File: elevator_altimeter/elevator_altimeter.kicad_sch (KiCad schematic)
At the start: 44 parts, among them J1 UART, J2 AVR-ICSP-TagConnect, J3 I2C, SW1 UserSW, U1 MPL3115A2, U2 NRF24L01_Breakout, U3 ATtiny1634-S, U4 MCP1711, U5 TP4056

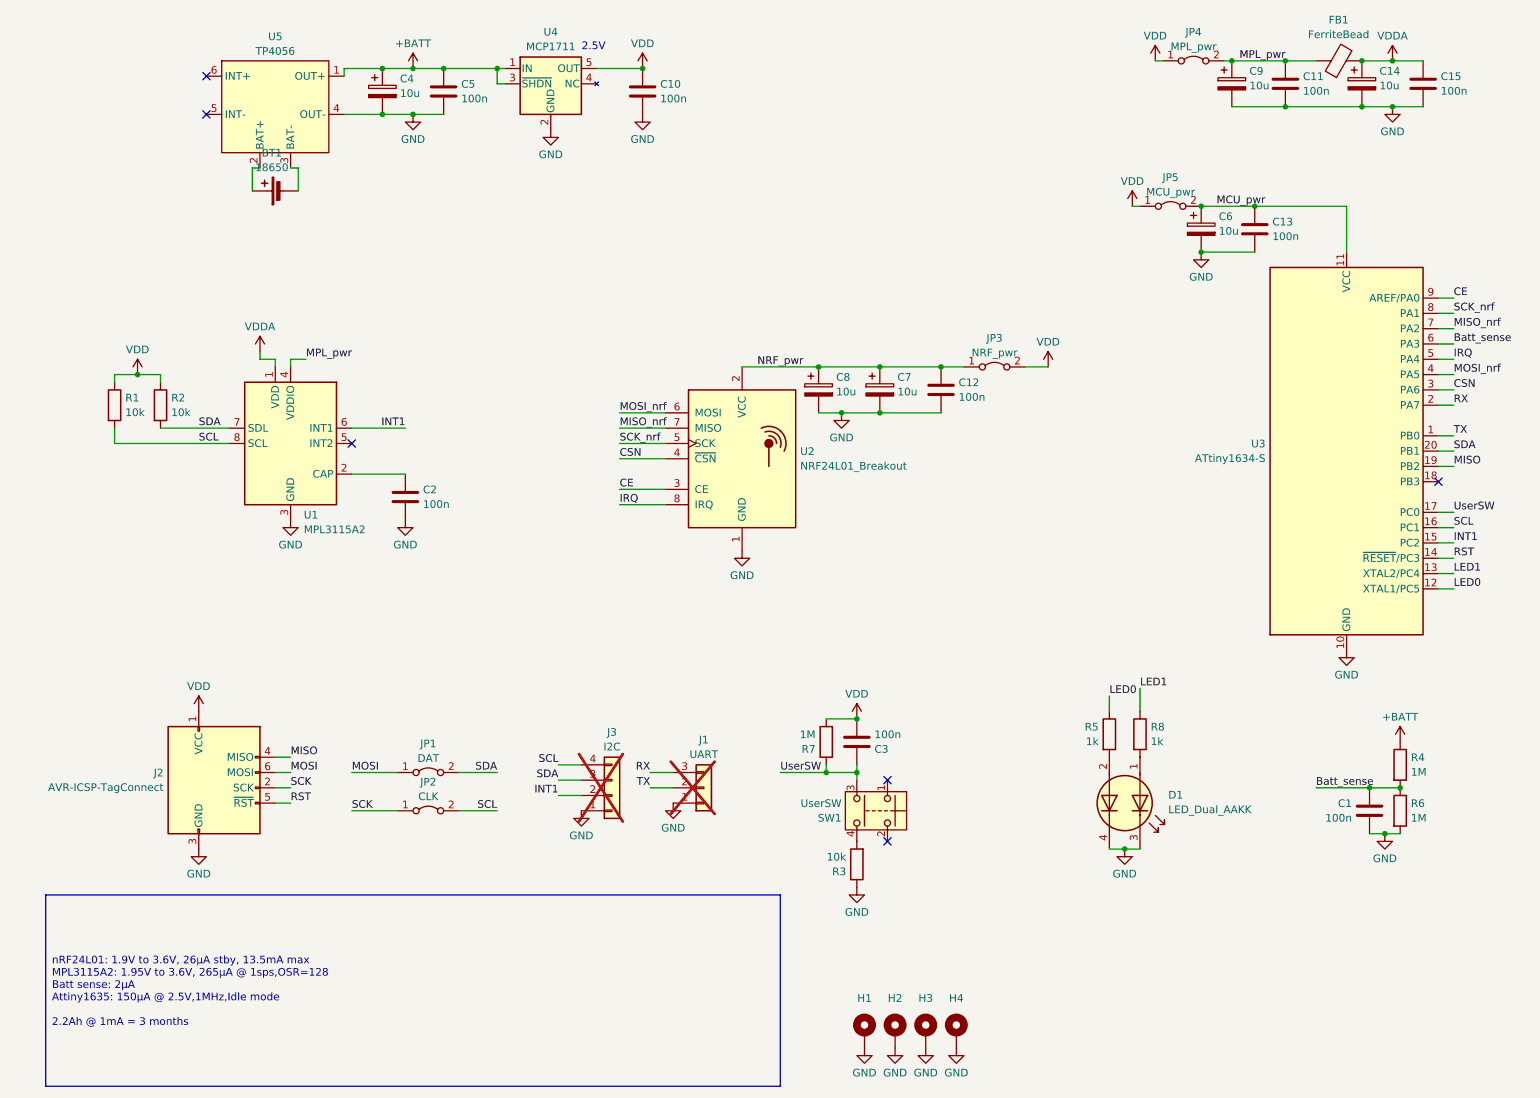
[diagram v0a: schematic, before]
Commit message: a
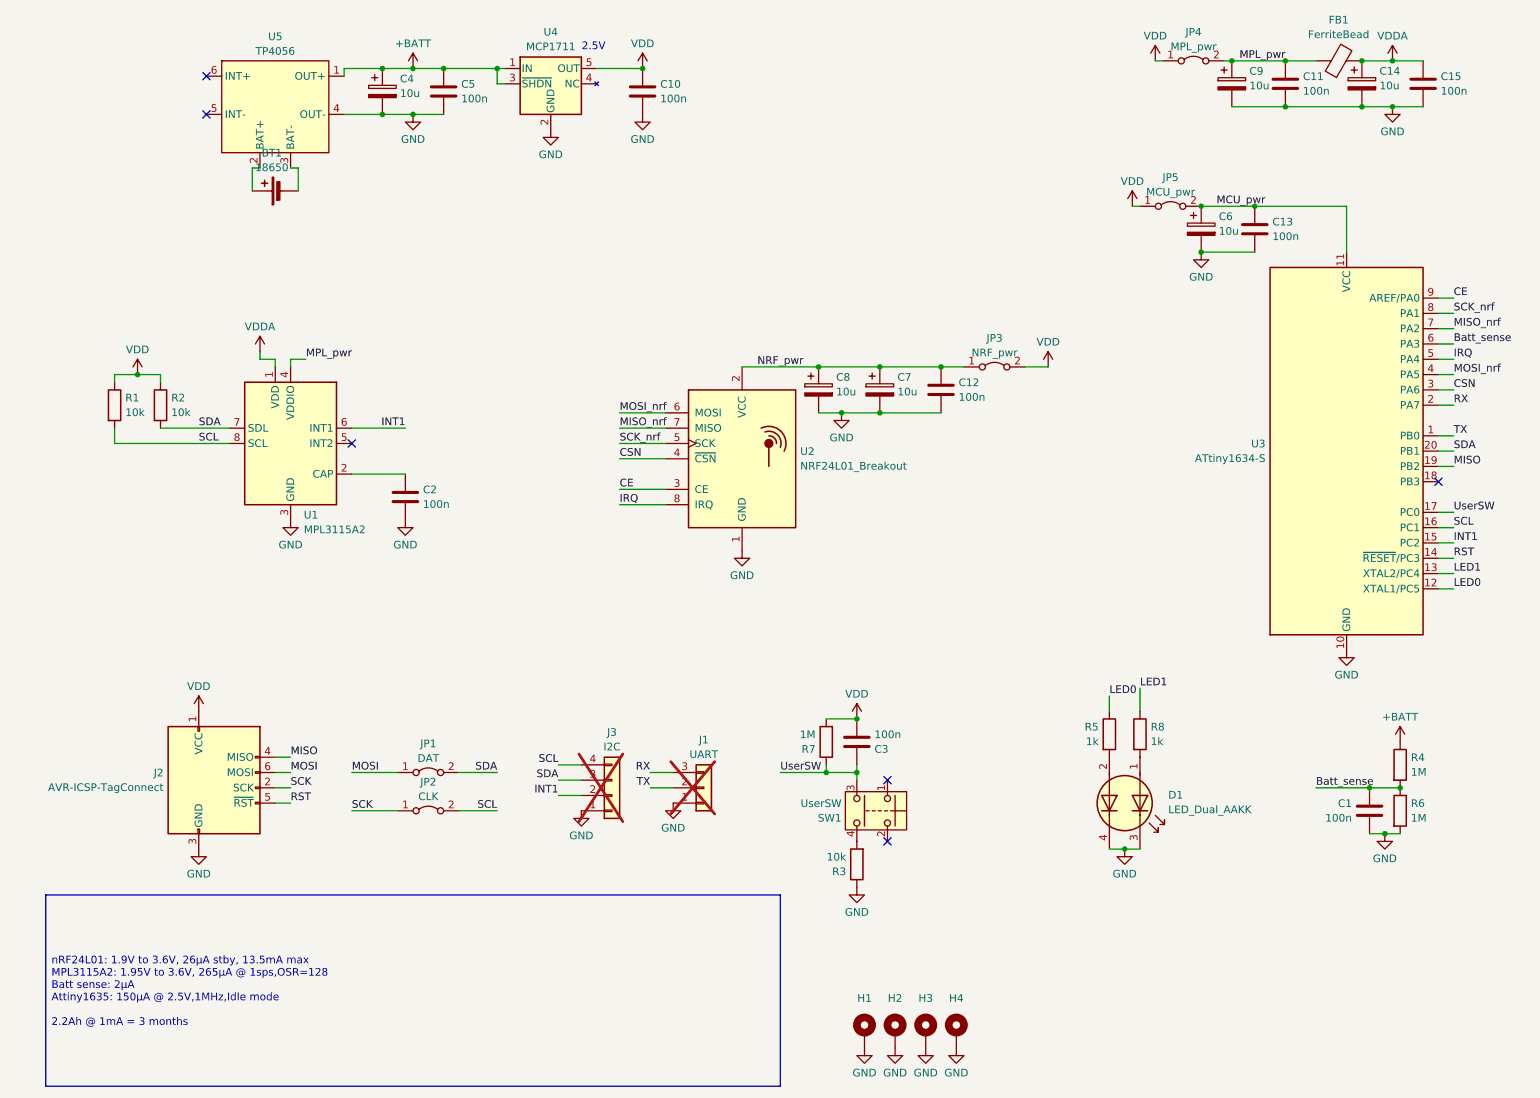
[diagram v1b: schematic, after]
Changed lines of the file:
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@@
 (kicad_sch
-	(version 20231120)
+	(version 20250114)
 	(generator "eeschema")
-	(generator_version "8.0")
+	(generator_version "9.0")
 	(paper "A4")
 	(title_block
@@
 		(company "Xavier Bourlot")
 	)
+	(text "2.5V"
+		(exclude_from_sim no)
+		(at 108.712 20.574 0)
+		(effects
+			(font
+				(size 1.27 1.27)
+			)
+		)
+	)
+	(text_box "nRF24L01: 1.9V to 3.6V, 26µA stby, 13.5mA max\nMPL3115A2: 1.95V to 3.6V, 265µA @ 1sps,OSR=128\nBatt sense: 2µA\nAttiny1635: 150µA @ 2.5V,1MHz,Idle mode\n\n2.2Ah @ 1mA = 3 months"
+		(exclude_from_sim no)
+		(at 17.78 161.29 0)
+		(size 121.92 31.75)
+		(margins 0.9525 0.9525 0.9525 0.9525)
+		(stroke
+			(width 0)
+			(type default)
+		)
+		(fill
+			(type color)
+			(color 255 255 194 1)
+		)
+		(effects
+			(font
+				(size 1.27 1.27)
+			)
+			(justify left)
+		)
+	)
 	(junction
 		(at 152.4 132.08)
@@
 		)
 	)
-	(text_box "nRF24L01: 1.9V to 3.6V, 26µA stby, 13.5mA max\nMPL3115A2: 1.95V to 3.6V, 265µA @ 1sps,OSR=128\nBatt sense: 2µA\nAttiny1635: 150µA @ 2.5V,1MHz,Idle mode\n\n2.2Ah @ 1mA = 3 months"
-		(exclude_from_sim no)
-		(at 17.78 161.29 0)
-		(size 121.92 31.75)
-		(stroke
-			(width 0)
-			(type default)
-		)
-		(fill
-			(type color)
-			(color 255 255 194 1)
-		)
-		(effects
-			(font
-				(size 1.27 1.27)
-			)
-			(justify left)
-		)
-	)
-	(text "2.5V"
-		(exclude_from_sim no)
-		(at 108.712 20.574 0)
-		(effects
-			(font
-				(size 1.27 1.27)
-			)
-		)
-	)
 	(label "SCL"
 		(at 251.46 100.33 0)
-		(fields_autoplaced yes)
 		(effects
 			(font
@@
 	(label "RX"
 		(at 251.46 80.01 0)
-		(fields_autoplaced yes)
 		(effects
 			(font
@@
 	(label "CE"
 		(at 251.46 62.23 0)
-		(fields_autoplaced yes)
 		(effects
 			(font
@@
 	(label "SDA"
 		(at 102.87 142.24 180)
-		(fields_autoplaced yes)
 		(effects
 			(font
@@
 	(label "MISO_nrf"
 		(at 113.03 83.82 0)
-		(fields_autoplaced yes)
 		(effects
 			(font
@@
 	(label "INT1"
 		(at 77.47 83.82 180)
-		(fields_autoplaced yes)
 		(effects
 			(font
@@
 	(label "SDA"
 		(at 92.71 140.97 180)
-		(fields_autoplaced yes)
 		(effects
 			(font
@@
 	(label "SCL"
 		(at 102.87 139.7 180)
-		(fields_autoplaced yes)
 		(effects
 			(font
@@
 	(label "MOSI_nrf"
 		(at 251.46 74.93 0)
-		(fields_autoplaced yes)
 		(effects
 			(font
@@
 	(label "MCU_pwr"
 		(at 212.09 46.99 0)
-		(fields_autoplaced yes)
 		(effects
 			(font
@@
 	(label "MPL_pwr"
 		(at 60.96 72.39 0)
-		(fields_autoplaced yes)
 		(effects
 			(font
@@
 	(label "LED1"
 		(at 251.46 107.95 0)
-		(fields_autoplaced yes)
 		(effects
 			(font
@@
 	(label "SCL"
 		(at 43.18 86.36 0)
-		(fields_autoplaced yes)
 		(effects
 			(font
@@
 	(label "TX"
 		(at 118.11 143.51 180)
-		(fields_autoplaced yes)
 		(effects
 			(font
@@
 	(label "MOSI"
 		(at 58.42 140.97 0)
-		(fields_autoplaced yes)
 		(effects
 			(font
@@
 	(label "Batt_sense"
 		(at 251.46 69.85 0)
-		(fields_autoplaced yes)
 		(effects
 			(font
@@
 	(label "LED0"
 		(at 251.46 110.49 0)
-		(fields_autoplaced yes)
 		(effects
 			(font
@@
 	(label "MISO"
 		(at 251.46 90.17 0)
-		(fields_autoplaced yes)
 		(effects
 			(font
@@
 	(label "RST"
 		(at 251.46 105.41 0)
-		(fields_autoplaced yes)
 		(effects
 			(font
@@
 	(label "SCK"
 		(at 68.58 147.32 0)
-		(fields_autoplaced yes)
 		(effects
 			(font
@@
 	(label "SCK"
 		(at 58.42 143.51 0)
-		(fields_autoplaced yes)
 		(effects
 			(font
@@
 	(label "MISO"
 		(at 58.42 138.43 0)
-		(fields_autoplaced yes)
 		(effects
 			(font
@@
 	(label "CE"
 		(at 113.03 93.98 0)
-		(fields_autoplaced yes)
 		(effects
 			(font
@@
 	(label "SCK_nrf"
 		(at 113.03 86.36 0)
-		(fields_autoplaced yes)
 		(effects
 			(font
@@
 	(label "RX"
 		(at 118.11 140.97 180)
-		(fields_autoplaced yes)
 		(effects
 			(font
@@
 	(label "MOSI_nrf"
 		(at 113.03 81.28 0)
-		(fields_autoplaced yes)
 		(effects
 			(font
@@
 	(label "Batt_sense"
 		(at 228.6 143.51 0)
-		(fields_autoplaced yes)
 		(effects
 			(font
@@
 	(label "RST"
 		(at 58.42 146.05 0)
-		(fields_autoplaced yes)
 		(effects
 			(font
@@
 	(label "SDA"
 		(at 43.18 83.82 0)
-		(fields_autoplaced yes)
 		(effects
 			(font
@@
 	(label "UserSW"
 		(at 251.46 97.79 0)
-		(fields_autoplaced yes)
 		(effects
 			(font
@@
 	(label "MOSI"
 		(at 68.58 140.97 0)
-		(fields_autoplaced yes)
 		(effects
 			(font
@@
 	(label "UserSW"
 		(at 139.7 140.97 0)
-		(fields_autoplaced yes)
 		(effects
 			(font
@@
 	(label "CSN"
 		(at 251.46 77.47 0)
-		(fields_autoplaced yes)
 		(effects
 			(font
@@
 	(label "NRF_pwr"
 		(at 135.89 73.66 0)
-		(fields_autoplaced yes)
 		(effects
 			(font
@@
 	(label "IRQ"
 		(at 251.46 72.39 0)
-		(fields_autoplaced yes)
 		(effects
 			(font
@@
 	(label "INT1"
 		(at 102.87 144.78 180)
-		(fields_autoplaced yes)
 		(effects
 			(font
@@
 	(label "IRQ"
 		(at 113.03 96.52 0)
-		(fields_autoplaced yes)
 		(effects
 			(font
@@
 	(label "SCL"
 		(at 92.71 147.32 180)
-		(fields_autoplaced yes)
 		(effects
 			(font
@@
 	(label "LED0"
 		(at 194.31 128.27 0)
-		(fields_autoplaced yes)
 		(effects
 			(font
@@
 	(label "SCK_nrf"
 		(at 251.46 64.77 0)
-		(fields_autoplaced yes)
 		(effects
 			(font
@@
 	(label "LED1"
 		(at 199.39 127 0)
-		(fields_autoplaced yes)
 		(effects
 			(font
@@
 	(label "TX"
 		(at 251.46 85.09 0)
-		(fields_autoplaced yes)
 		(effects
 			(font
@@
 	(label "INT1"
 		(at 251.46 102.87 0)
-		(fields_autoplaced yes)
 		(effects
 			(font
@@
 	(label "MISO_nrf"
 		(at 251.46 67.31 0)
-		(fields_autoplaced yes)
 		(effects
 			(font
@@
 	(label "SDA"
 		(at 251.46 87.63 0)
-		(fields_autoplaced yes)
 		(effects
 			(font
@@
 	(label "CSN"
 		(at 113.03 88.9 0)
-		(fields_autoplaced yes)
 		(effects
 			(font
@@
 	(label "MPL_pwr"
 		(at 215.9 22.86 0)
-		(fields_autoplaced yes)
 		(effects
 			(font
@@
 		)
 		(instances
-			(project ""
+			(project "elevator_altimeter"
 				(path "/acf46b34-b9a0-4f2e-b08a-347c81969a5c"
 					(reference "JP3")
@@
 		)
 	)
+	(embedded_fonts no)
 )
